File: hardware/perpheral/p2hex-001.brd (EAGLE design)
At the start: 89 x 51 mm, 2 parts

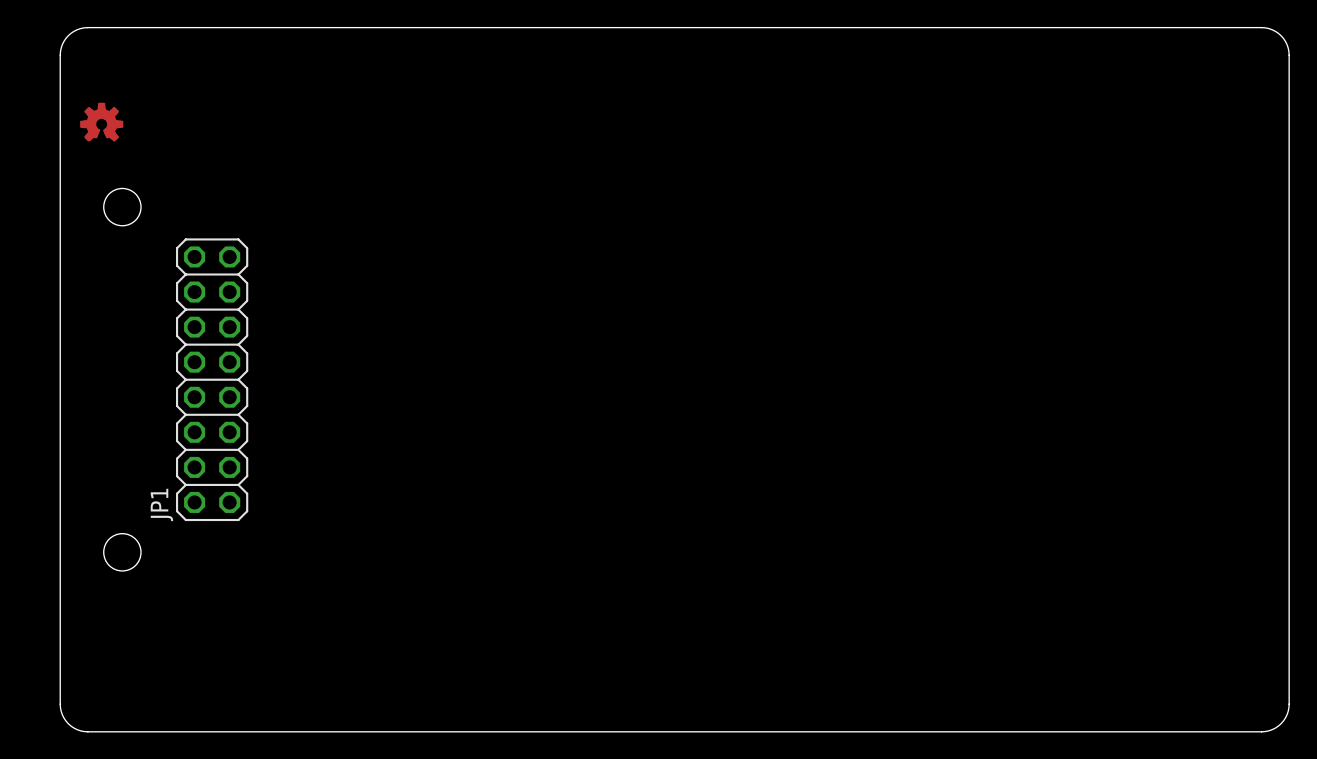
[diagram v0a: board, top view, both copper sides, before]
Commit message: First try.
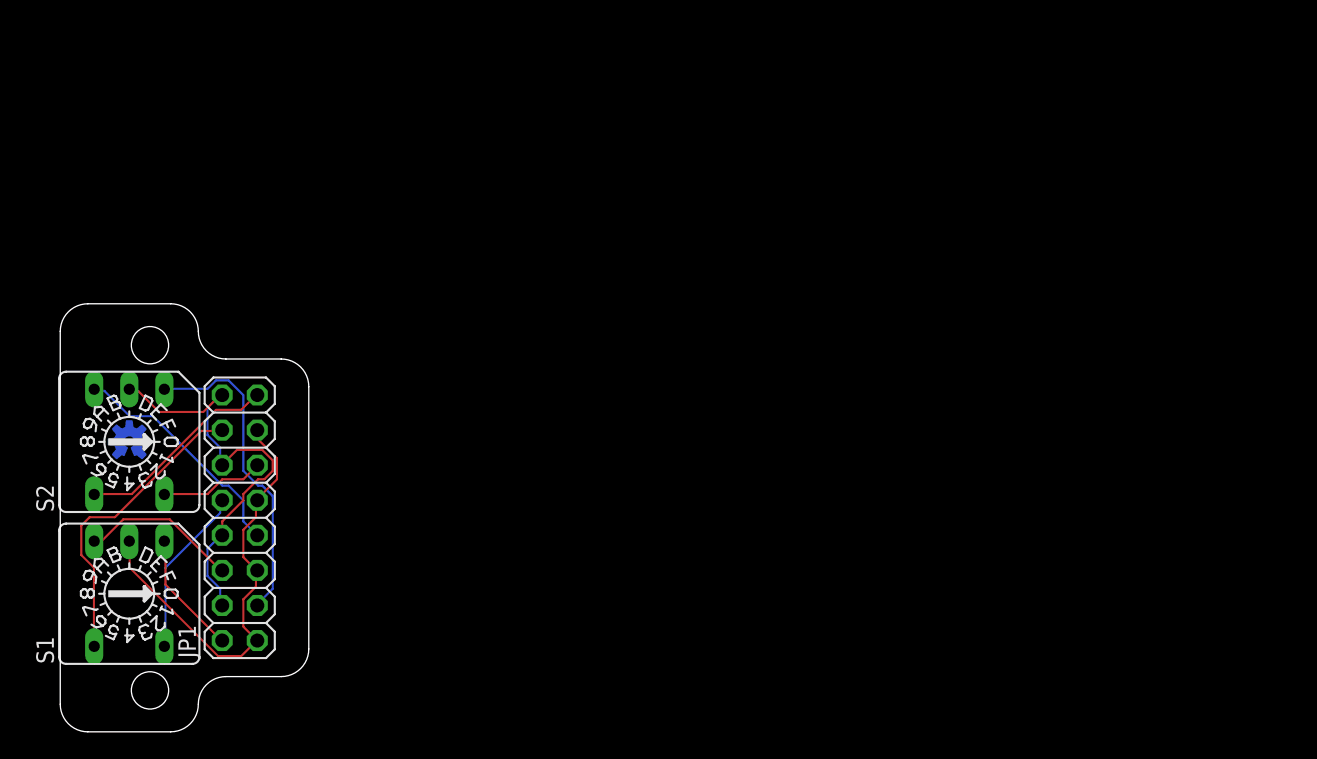
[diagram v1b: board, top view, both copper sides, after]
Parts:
- added S1, S2: (no value), switch-dil:A1353HEX
- moved LOGO1 23.1 mm to (5.00, 21.0), flipped to the bottom
- moved JP1 10.2 mm to (13.0, 15.5)
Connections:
- new net ANLG0: JP1.3, S2.1
- new net ANLG1: JP1.7, S2.4
- new net ANLG2: JP1.11, S2.8
- new net ANLG3: JP1.15, S2.2
- new net DTCT0: JP1.2, S1.1
- new net DTCT1: JP1.6, S1.4
- new net DTCT2: JP1.10, S1.8
- new net DTCT3: JP1.14, S1.2
- new net GND: JP1.1, JP1.13, JP1.5, JP1.9, S1.C
- new net VCC: JP1.12, JP1.16, JP1.4, JP1.8, S2.C
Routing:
- net GND: track 0.00 -> 32.4 mm
- net VCC: track 0.00 -> 31.7 mm
- net ANLG0: track 0.00 -> 23.2 mm
- net DTCT3: track 0.00 -> 22.2 mm
- net ANLG1: track 0.00 -> 17.1 mm
- net ANLG3: track 0.00 -> 14.8 mm
- net DTCT2: track 0.00 -> 12.4 mm
- net DTCT1: track 0.00 -> 11.4 mm
- net DTCT0: track 0.00 -> 8.95 mm
- net ANLG2: track 0.00 -> 7.60 mm
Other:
- board size 89 x 51 mm -> 18 x 31 mm
- board text added: "2"
- board text added: "4"
- board text added: "8"
